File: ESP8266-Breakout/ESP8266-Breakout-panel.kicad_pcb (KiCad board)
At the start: 2 copper layers, 98.8 x 97.2 mm, 258 parts, among them J101 Conn_01x09_Female, J102 Conn_01x09_Female, J501 FTDI, SW501 Flash, SW502 RST, U101 AMS1117-3.3, U501 ESP-12F

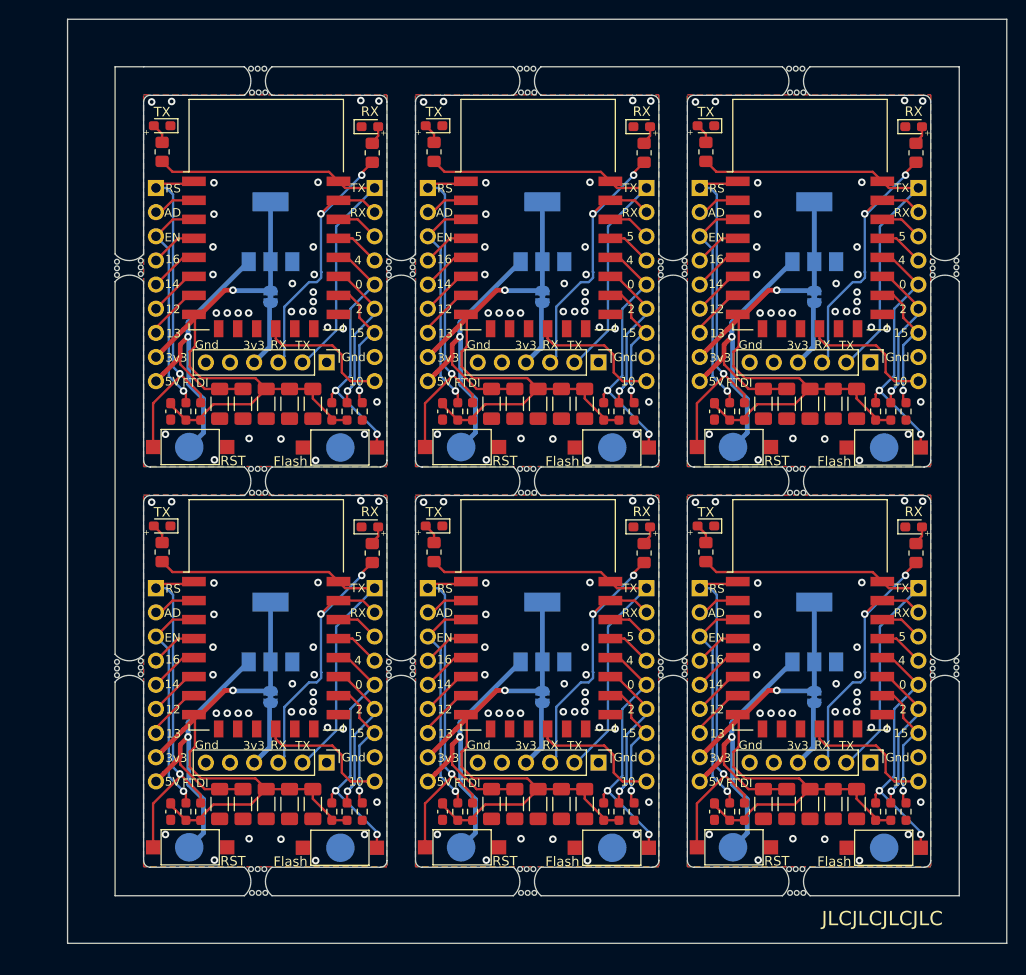
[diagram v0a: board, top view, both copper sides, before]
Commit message: Release 2
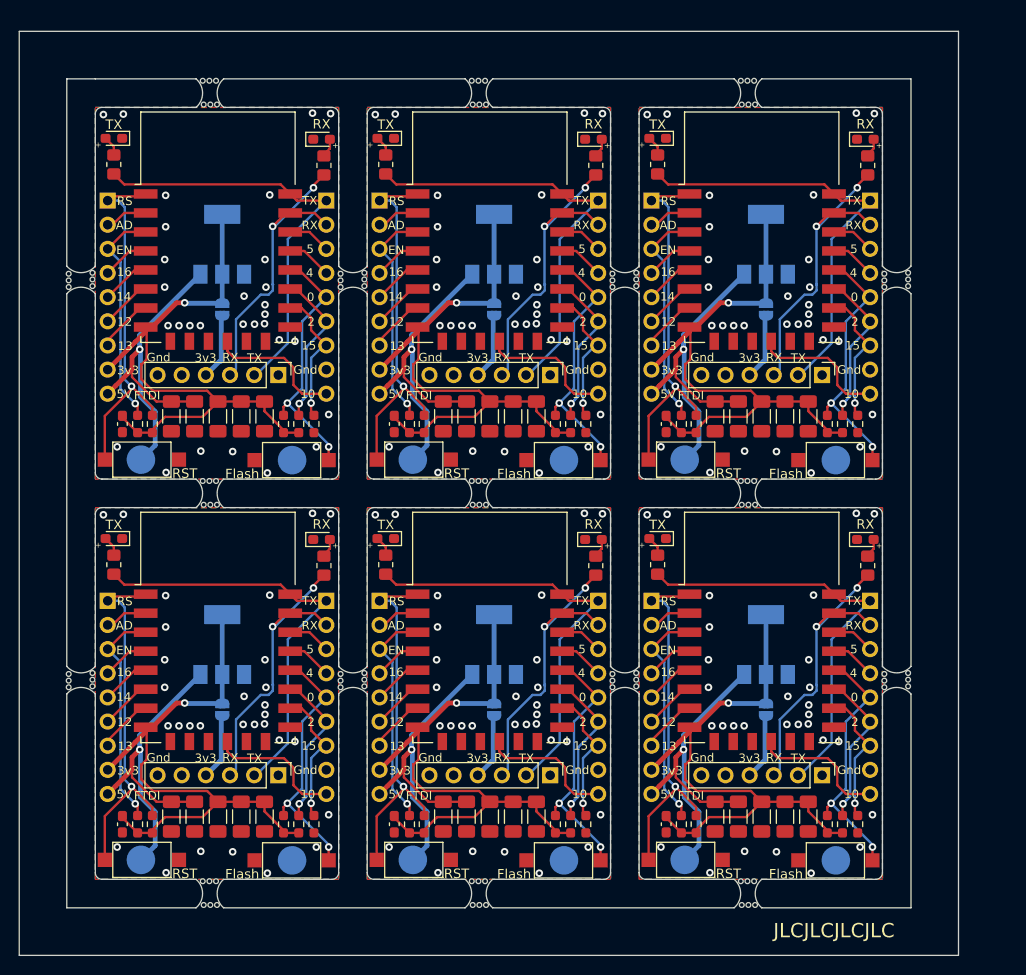
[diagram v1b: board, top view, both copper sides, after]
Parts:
- removed the C101 at (177.6, 129.2)
- removed the C101 at (148.9, 129.2)
- removed the C101 at (120.3, 129.2)
- removed the C101 at (177.6, 87.0)
- removed the C101 at (148.9, 87.0)
- removed the C101 at (120.3, 87.0)
- removed the C102 at (175.1, 129.2)
- removed the C102 at (146.5, 129.2)
- removed the C102 at (117.9, 129.2)
- removed the C102 at (175.1, 87.0)
- removed the C102 at (146.5, 87.0)
- removed the C102 at (117.9, 87.0)
- removed the C103 at (182.4, 129.2)
- removed the C103 at (153.8, 129.2)
- removed the C103 at (125.2, 129.2)
- removed the C103 at (182.4, 87.0)
- removed the C103 at (153.8, 87.0)
- removed the C103 at (125.2, 87.0)
- removed the C104 at (184.9, 129.2)
- removed the C104 at (156.3, 129.2)
- removed the C104 at (127.7, 129.2)
- removed the C104 at (184.9, 87.0)
- removed the C104 at (156.3, 87.0)
- removed the C104 at (127.7, 87.0)
- removed the C501 at (169.9, 129.9)
- removed the C501 at (141.3, 129.9)
- removed the C501 at (112.8, 129.9)
- removed the C501 at (169.9, 87.8)
- removed the C501 at (141.3, 87.8)
- removed the C501 at (112.8, 87.8)
- removed the C502 at (180.0, 129.2)
- removed the C502 at (151.4, 129.2)
- removed the C502 at (122.8, 129.2)
- removed the C502 at (180.0, 87.0)
- removed the C502 at (151.4, 87.0)
- removed the C502 at (122.8, 87.0)
- removed the D501 at (169.1, 99.9)
- removed the D501 at (140.4, 99.9)
- removed the D501 at (111.8, 99.9)
- removed the D501 at (169.1, 57.8)
- removed the D501 at (140.4, 57.8)
- removed the D501 at (111.8, 57.8)
- removed the D502 at (190.9, 100.0)
- removed the D502 at (162.3, 100.0)
- removed the D502 at (133.7, 100.0)
- removed the D502 at (190.9, 57.9)
- removed the D502 at (162.3, 57.9)
- removed the D502 at (133.7, 57.9)
- removed the J101 at (168.4, 106.5)
- removed the J101 at (139.8, 106.5)
- removed the J101 at (111.2, 106.5)
- removed the J101 at (168.4, 64.3)
- removed the J101 at (139.8, 64.3)
- removed the J101 at (111.2, 64.3)
- removed the J102 at (191.4, 106.5)
- removed the J102 at (162.8, 106.5)
- removed the J102 at (134.2, 106.5)
- removed the J102 at (191.4, 64.3)
- removed the J102 at (162.8, 64.3)
- removed the J102 at (134.2, 64.3)
- removed the J501 at (186.3, 124.8)
- removed the J501 at (157.8, 124.8)
- removed the J501 at (129.2, 124.8)
- removed the J501 at (186.3, 82.7)
- removed the J501 at (157.8, 82.7)
- removed the J501 at (129.2, 82.7)
- removed the JP501 at (180.4, 117.9)
- removed the JP501 at (151.8, 117.9)
- removed the JP501 at (123.2, 117.9)
- removed the JP501 at (180.4, 75.8)
- removed the JP501 at (151.8, 75.8)
- removed the JP501 at (123.2, 75.8)
- removed the R501 at (186.9, 129.9)
- removed the R501 at (158.3, 129.9)
- removed the R501 at (129.7, 129.9)
- removed the R501 at (186.9, 87.8)
- removed the R501 at (158.3, 87.8)
- removed the R501 at (129.7, 87.8)
- removed the R502 at (173.1, 129.9)
- removed the R502 at (144.5, 129.9)
- removed the R502 at (115.9, 129.9)
- removed the R502 at (173.1, 87.8)
- removed the R502 at (144.5, 87.8)
- removed the R502 at (115.9, 87.8)
- removed the R503 at (171.6, 129.9)
- removed the R503 at (142.9, 129.9)
- removed the R503 at (114.3, 129.9)
- removed the R503 at (171.6, 87.8)
- removed the R503 at (142.9, 87.8)
- removed the R503 at (114.3, 87.8)
- removed the R504 at (169.1, 102.7)
- removed the R504 at (140.4, 102.7)
- removed the R504 at (111.8, 102.7)
- removed the R504 at (169.1, 60.5)
- removed the R504 at (140.4, 60.5)
- removed the R504 at (111.8, 60.5)
- removed the R505 at (188.5, 129.9)
- removed the R505 at (159.9, 129.9)
- removed the R505 at (131.3, 129.9)
- removed the R505 at (188.5, 87.8)
- removed the R505 at (159.9, 87.8)
- removed the R505 at (131.3, 87.8)
- removed the R506 at (190.1, 129.9)
- removed the R506 at (161.5, 129.9)
- removed the R506 at (132.9, 129.9)
- removed the R506 at (190.1, 87.8)
- removed the R506 at (161.5, 87.8)
- removed the R506 at (132.9, 87.8)
- removed the R507 at (191.2, 102.8)
- removed the R507 at (162.6, 102.8)
- removed the R507 at (133.9, 102.8)
- removed the R507 at (191.2, 60.6)
- removed the R507 at (162.6, 60.6)
- removed the R507 at (133.9, 60.6)
- removed the REF** at (179.9, 100.3)
- removed the REF** at (109.6, 115.5)
- removed the REF** at (121.3, 96.4)
- removed the REF** at (177.9, 54.3)
- removed the REF** at (149.6, 54.3)
- removed the REF** at (122.0, 54.3)
- removed the REF** at (122.7, 54.3)
- removed the REF** at (121.3, 54.3)
- removed the REF** at (122.6, 51.8)
- removed the REF** at (121.9, 51.8)
- removed the REF** at (121.2, 51.8)
- removed the REF** at (195.4, 73.4)
- removed the REF** at (166.8, 73.4)
- removed the REF** at (138.2, 73.4)
- removed the REF** at (192.9, 115.6)
- removed the REF** at (164.3, 115.6)
- removed the REF** at (135.7, 115.6)
- removed the REF** at (107.1, 115.6)
- removed the REF** at (192.9, 73.5)
- removed the REF** at (164.3, 73.5)
- removed the REF** at (151.3, 100.3)
- removed the REF** at (135.7, 73.5)
- removed the REF** at (192.9, 114.9)
- removed the REF** at (164.3, 114.9)
- removed the REF** at (135.7, 114.9)
- removed the REF** at (107.1, 114.9)
- removed the REF** at (192.9, 72.8)
- removed the REF** at (164.3, 72.8)
- removed the REF** at (135.7, 72.8)
- removed the REF** at (192.9, 114.2)
- removed the REF** at (164.3, 114.2)
- removed the REF** at (122.7, 100.3)
- removed the REF** at (135.7, 114.2)
- removed the REF** at (107.1, 114.2)
- removed the REF** at (192.9, 72.1)
- removed the REF** at (164.3, 72.1)
- removed the REF** at (135.7, 72.1)
- removed the REF** at (195.4, 114.1)
- removed the REF** at (166.8, 114.1)
- removed the REF** at (138.2, 114.1)
- removed the REF** at (109.6, 114.1)
- removed the REF** at (195.4, 72.0)
- removed the REF** at (179.9, 58.2)
- removed the REF** at (166.8, 72.0)
- removed the REF** at (138.2, 72.0)
- removed the REF** at (195.4, 114.8)
- removed the REF** at (166.8, 114.8)
- removed the REF** at (138.2, 114.8)
- removed the REF** at (109.6, 114.8)
- removed the REF** at (195.4, 72.7)
- removed the REF** at (166.8, 72.7)
- removed the REF** at (138.2, 72.7)
- removed the REF** at (109.6, 72.7)
- removed the REF** at (151.3, 58.2)
- removed the REF** at (109.6, 72.0)
- removed the REF** at (107.1, 72.8)
- removed the REF** at (107.1, 72.1)
- removed the REF** at (107.1, 73.5)
- removed the REF** at (109.6, 73.4)
- removed the REF** at (178.6, 138.5)
- removed the REF** at (150.3, 138.5)
- removed the REF** at (122.0, 138.5)
- removed the REF** at (178.6, 96.4)
- removed the REF** at (150.3, 96.4)
- removed the REF** at (122.7, 58.2)
- removed the REF** at (122.0, 96.4)
- removed the REF** at (178.6, 54.3)
- removed the REF** at (150.3, 54.3)
- removed the REF** at (179.3, 138.5)
- removed the REF** at (151.0, 138.5)
- removed the REF** at (122.7, 138.5)
- removed the REF** at (179.3, 96.4)
- removed the REF** at (151.0, 96.4)
- removed the REF** at (122.7, 96.4)
- removed the REF** at (179.3, 54.3)
- removed the REF** at (195.4, 115.5)
- removed the REF** at (151.0, 54.3)
- removed the REF** at (178.5, 136.0)
- removed the REF** at (150.2, 136.0)
- removed the REF** at (121.9, 136.0)
- removed the REF** at (178.5, 93.9)
- removed the REF** at (150.2, 93.9)
- removed the REF** at (121.9, 93.9)
- removed the REF** at (178.5, 51.8)
- removed the REF** at (150.2, 51.8)
- removed the REF** at (179.2, 136.0)
- removed the REF** at (166.8, 115.5)
- removed the REF** at (150.9, 136.0)
- removed the REF** at (122.6, 136.0)
- removed the REF** at (179.2, 93.9)
- removed the REF** at (150.9, 93.9)
- removed the REF** at (122.6, 93.9)
- removed the REF** at (179.2, 51.8)
- removed the REF** at (150.9, 51.8)
- removed the REF** at (177.8, 136.0)
- removed the REF** at (149.5, 136.0)
- removed the REF** at (121.2, 136.0)
- removed the REF** at (138.2, 115.5)
- removed the REF** at (177.8, 93.9)
- removed the REF** at (149.5, 93.9)
- removed the REF** at (121.2, 93.9)
- removed the REF** at (177.8, 51.8)
- removed the REF** at (149.5, 51.8)
- removed the REF** at (177.9, 138.5)
- removed the REF** at (149.6, 138.5)
- removed the REF** at (121.3, 138.5)
- removed the REF** at (177.9, 96.4)
- removed the REF** at (149.6, 96.4)
- removed the SW501 at (187.8, 133.8)
- removed the SW501 at (159.2, 133.8)
- removed the SW501 at (130.6, 133.8)
- removed the SW501 at (187.8, 91.7)
- removed the SW501 at (159.2, 91.7)
- removed the SW501 at (130.6, 91.7)
- removed the SW502 at (172.0, 133.7)
- removed the SW502 at (143.4, 133.7)
- removed the SW502 at (114.8, 133.7)
- removed the SW502 at (172.0, 91.6)
- removed the SW502 at (143.4, 91.6)
- removed the SW502 at (114.8, 91.6)
- removed the TP101 at (171.9, 133.7)
- removed the TP101 at (143.3, 133.7)
- removed the TP101 at (114.7, 133.7)
- removed the TP101 at (171.9, 91.6)
- removed the TP101 at (143.3, 91.6)
- removed the TP101 at (114.7, 91.6)
- removed the TP102 at (187.8, 133.8)
- removed the TP102 at (159.2, 133.8)
- removed the TP102 at (130.6, 133.8)
- removed the TP102 at (187.8, 91.7)
- removed the TP102 at (159.2, 91.7)
- removed the TP102 at (130.6, 91.7)
- removed the U101 at (180.4, 111.0)
- removed the U101 at (151.8, 111.0)
- removed the U101 at (123.2, 111.0)
- removed the U101 at (180.4, 69.0)
- removed the U101 at (151.8, 69.0)
- removed the U101 at (123.2, 69.0)
- removed the U501 at (180.0, 109.2)
- removed the U501 at (151.4, 109.2)
- removed the U501 at (122.8, 109.2)
- removed the U501 at (180.0, 67.2)
- removed the U501 at (151.4, 67.2)
- removed the U501 at (122.8, 67.2)
- added C101: 10uF, Capacitor_SMD:C_1206_3216Metric_Pad1.33x1.80mm_HandSolder, F.Cu at (172.5, 130.5)
- added C101: 10uF, Capacitor_SMD:C_1206_3216Metric_Pad1.33x1.80mm_HandSolder, F.Cu at (143.9, 130.5)
- added C101: 10uF, Capacitor_SMD:C_1206_3216Metric_Pad1.33x1.80mm_HandSolder, F.Cu at (115.3, 130.5)
- added C101: 10uF, Capacitor_SMD:C_1206_3216Metric_Pad1.33x1.80mm_HandSolder, F.Cu at (172.5, 88.4)
- added C101: 10uF, Capacitor_SMD:C_1206_3216Metric_Pad1.33x1.80mm_HandSolder, F.Cu at (143.9, 88.4)
- added C101: 10uF, Capacitor_SMD:C_1206_3216Metric_Pad1.33x1.80mm_HandSolder, F.Cu at (115.3, 88.4)
- added C102: 100nF, Capacitor_SMD:C_1206_3216Metric_Pad1.33x1.80mm_HandSolder, F.Cu at (170.0, 130.5)
- added C102: 100nF, Capacitor_SMD:C_1206_3216Metric_Pad1.33x1.80mm_HandSolder, F.Cu at (141.4, 130.5)
- added C102: 100nF, Capacitor_SMD:C_1206_3216Metric_Pad1.33x1.80mm_HandSolder, F.Cu at (112.8, 130.5)
- added C102: 100nF, Capacitor_SMD:C_1206_3216Metric_Pad1.33x1.80mm_HandSolder, F.Cu at (170.0, 88.4)
- added C102: 100nF, Capacitor_SMD:C_1206_3216Metric_Pad1.33x1.80mm_HandSolder, F.Cu at (141.4, 88.4)
- added C102: 100nF, Capacitor_SMD:C_1206_3216Metric_Pad1.33x1.80mm_HandSolder, F.Cu at (112.8, 88.4)
- added C103: 100nF, Capacitor_SMD:C_1206_3216Metric_Pad1.33x1.80mm_HandSolder, F.Cu at (177.4, 130.5)
- added C103: 100nF, Capacitor_SMD:C_1206_3216Metric_Pad1.33x1.80mm_HandSolder, F.Cu at (148.8, 130.5)
- added C103: 100nF, Capacitor_SMD:C_1206_3216Metric_Pad1.33x1.80mm_HandSolder, F.Cu at (120.2, 130.5)
- added C103: 100nF, Capacitor_SMD:C_1206_3216Metric_Pad1.33x1.80mm_HandSolder, F.Cu at (177.4, 88.4)
- added C103: 100nF, Capacitor_SMD:C_1206_3216Metric_Pad1.33x1.80mm_HandSolder, F.Cu at (148.8, 88.4)
- added C103: 100nF, Capacitor_SMD:C_1206_3216Metric_Pad1.33x1.80mm_HandSolder, F.Cu at (120.2, 88.4)
- added C104: 10uF, Capacitor_SMD:C_1206_3216Metric_Pad1.33x1.80mm_HandSolder, F.Cu at (179.8, 130.5)
- added C104: 10uF, Capacitor_SMD:C_1206_3216Metric_Pad1.33x1.80mm_HandSolder, F.Cu at (151.2, 130.5)
- added C104: 10uF, Capacitor_SMD:C_1206_3216Metric_Pad1.33x1.80mm_HandSolder, F.Cu at (122.6, 130.5)
- added C104: 10uF, Capacitor_SMD:C_1206_3216Metric_Pad1.33x1.80mm_HandSolder, F.Cu at (179.8, 88.4)
- added C104: 10uF, Capacitor_SMD:C_1206_3216Metric_Pad1.33x1.80mm_HandSolder, F.Cu at (151.2, 88.4)
- added C104: 10uF, Capacitor_SMD:C_1206_3216Metric_Pad1.33x1.80mm_HandSolder, F.Cu at (122.6, 88.4)
- added C501: 0.1uF, Capacitor_SMD:C_0603_1608Metric_Pad1.08x0.95mm_HandSolder, F.Cu at (164.9, 131.3)
- added C501: 0.1uF, Capacitor_SMD:C_0603_1608Metric_Pad1.08x0.95mm_HandSolder, F.Cu at (136.3, 131.3)
- added C501: 0.1uF, Capacitor_SMD:C_0603_1608Metric_Pad1.08x0.95mm_HandSolder, F.Cu at (107.7, 131.3)
- added C501: 0.1uF, Capacitor_SMD:C_0603_1608Metric_Pad1.08x0.95mm_HandSolder, F.Cu at (164.9, 89.2)
- added C501: 0.1uF, Capacitor_SMD:C_0603_1608Metric_Pad1.08x0.95mm_HandSolder, F.Cu at (136.3, 89.2)
- added C501: 0.1uF, Capacitor_SMD:C_0603_1608Metric_Pad1.08x0.95mm_HandSolder, F.Cu at (107.7, 89.2)
- added C502: 47uF, Capacitor_SMD:C_1206_3216Metric_Pad1.33x1.80mm_HandSolder, F.Cu at (174.9, 130.5)
- added C502: 47uF, Capacitor_SMD:C_1206_3216Metric_Pad1.33x1.80mm_HandSolder, F.Cu at (146.3, 130.5)
- added C502: 47uF, Capacitor_SMD:C_1206_3216Metric_Pad1.33x1.80mm_HandSolder, F.Cu at (117.7, 130.5)
- added C502: 47uF, Capacitor_SMD:C_1206_3216Metric_Pad1.33x1.80mm_HandSolder, F.Cu at (174.9, 88.4)
- added C502: 47uF, Capacitor_SMD:C_1206_3216Metric_Pad1.33x1.80mm_HandSolder, F.Cu at (146.3, 88.4)
- added C502: 47uF, Capacitor_SMD:C_1206_3216Metric_Pad1.33x1.80mm_HandSolder, F.Cu at (117.7, 88.4)
- added D501: TX, LED_SMD:LED_0603_1608Metric_Pad1.05x0.95mm_HandSolder, F.Cu at (164.0, 101.2)
- added D501: TX, LED_SMD:LED_0603_1608Metric_Pad1.05x0.95mm_HandSolder, F.Cu at (135.4, 101.2)
- added D501: TX, LED_SMD:LED_0603_1608Metric_Pad1.05x0.95mm_HandSolder, F.Cu at (106.8, 101.2)
- added D501: TX, LED_SMD:LED_0603_1608Metric_Pad1.05x0.95mm_HandSolder, F.Cu at (164.0, 59.1)
- added D501: TX, LED_SMD:LED_0603_1608Metric_Pad1.05x0.95mm_HandSolder, F.Cu at (135.4, 59.1)
- added D501: TX, LED_SMD:LED_0603_1608Metric_Pad1.05x0.95mm_HandSolder, F.Cu at (106.8, 59.1)
- added D502: RX, LED_SMD:LED_0603_1608Metric_Pad1.05x0.95mm_HandSolder, F.Cu at (185.8, 101.3)
- added D502: RX, LED_SMD:LED_0603_1608Metric_Pad1.05x0.95mm_HandSolder, F.Cu at (157.2, 101.3)
- added D502: RX, LED_SMD:LED_0603_1608Metric_Pad1.05x0.95mm_HandSolder, F.Cu at (128.6, 101.3)
- added D502: RX, LED_SMD:LED_0603_1608Metric_Pad1.05x0.95mm_HandSolder, F.Cu at (185.8, 59.2)
- added D502: RX, LED_SMD:LED_0603_1608Metric_Pad1.05x0.95mm_HandSolder, F.Cu at (157.2, 59.2)
- added D502: RX, LED_SMD:LED_0603_1608Metric_Pad1.05x0.95mm_HandSolder, F.Cu at (128.6, 59.2)
- added J101: Conn_01x09_Female, Custom:PinHeader_1x09_P2.54mm_Vertical_without_silkscrean, F.Cu at (163.3, 107.8)
- added J101: Conn_01x09_Female, Custom:PinHeader_1x09_P2.54mm_Vertical_without_silkscrean, F.Cu at (134.7, 107.8)
- added J101: Conn_01x09_Female, Custom:PinHeader_1x09_P2.54mm_Vertical_without_silkscrean, F.Cu at (106.1, 107.8)
- added J101: Conn_01x09_Female, Custom:PinHeader_1x09_P2.54mm_Vertical_without_silkscrean, F.Cu at (163.3, 65.7)
- added J101: Conn_01x09_Female, Custom:PinHeader_1x09_P2.54mm_Vertical_without_silkscrean, F.Cu at (134.7, 65.7)
- added J101: Conn_01x09_Female, Custom:PinHeader_1x09_P2.54mm_Vertical_without_silkscrean, F.Cu at (106.1, 65.7)
- added J102: Conn_01x09_Female, Custom:PinHeader_1x09_P2.54mm_Vertical_without_silkscrean, F.Cu at (186.3, 107.8)
- added J102: Conn_01x09_Female, Custom:PinHeader_1x09_P2.54mm_Vertical_without_silkscrean, F.Cu at (157.7, 107.8)
- added J102: Conn_01x09_Female, Custom:PinHeader_1x09_P2.54mm_Vertical_without_silkscrean, F.Cu at (129.1, 107.8)
- added J102: Conn_01x09_Female, Custom:PinHeader_1x09_P2.54mm_Vertical_without_silkscrean, F.Cu at (186.3, 65.7)
- added J102: Conn_01x09_Female, Custom:PinHeader_1x09_P2.54mm_Vertical_without_silkscrean, F.Cu at (157.7, 65.7)
- added J102: Conn_01x09_Female, Custom:PinHeader_1x09_P2.54mm_Vertical_without_silkscrean, F.Cu at (129.1, 65.7)
- added J501: FTDI, Connector_PinHeader_2.54mm:PinHeader_1x06_P2.54mm_Vertical, F.Cu at (181.3, 126.1)
- added J501: FTDI, Connector_PinHeader_2.54mm:PinHeader_1x06_P2.54mm_Vertical, F.Cu at (152.7, 126.1)
- added J501: FTDI, Connector_PinHeader_2.54mm:PinHeader_1x06_P2.54mm_Vertical, F.Cu at (124.1, 126.1)
- added J501: FTDI, Connector_PinHeader_2.54mm:PinHeader_1x06_P2.54mm_Vertical, F.Cu at (181.3, 84.0)
- added J501: FTDI, Connector_PinHeader_2.54mm:PinHeader_1x06_P2.54mm_Vertical, F.Cu at (152.7, 84.0)
- added J501: FTDI, Connector_PinHeader_2.54mm:PinHeader_1x06_P2.54mm_Vertical, F.Cu at (124.1, 84.0)
- added JP501: Power, Jumper:SolderJumper-2_P1.3mm_Open_RoundedPad1.0x1.5mm, B.Cu at (175.4, 119.2)
- added JP501: Power, Jumper:SolderJumper-2_P1.3mm_Open_RoundedPad1.0x1.5mm, B.Cu at (146.8, 119.2)
- added JP501: Power, Jumper:SolderJumper-2_P1.3mm_Open_RoundedPad1.0x1.5mm, B.Cu at (118.2, 119.2)
- added JP501: Power, Jumper:SolderJumper-2_P1.3mm_Open_RoundedPad1.0x1.5mm, B.Cu at (175.4, 77.1)
- added JP501: Power, Jumper:SolderJumper-2_P1.3mm_Open_RoundedPad1.0x1.5mm, B.Cu at (146.8, 77.1)
- added JP501: Power, Jumper:SolderJumper-2_P1.3mm_Open_RoundedPad1.0x1.5mm, B.Cu at (118.2, 77.1)
- added R501: 10K, Resistor_SMD:R_0603_1608Metric_Pad0.98x0.95mm_HandSolder, F.Cu at (181.8, 131.3)
- added R501: 10K, Resistor_SMD:R_0603_1608Metric_Pad0.98x0.95mm_HandSolder, F.Cu at (153.2, 131.3)
- added R501: 10K, Resistor_SMD:R_0603_1608Metric_Pad0.98x0.95mm_HandSolder, F.Cu at (124.6, 131.3)
- added R501: 10K, Resistor_SMD:R_0603_1608Metric_Pad0.98x0.95mm_HandSolder, F.Cu at (181.8, 89.2)
- added R501: 10K, Resistor_SMD:R_0603_1608Metric_Pad0.98x0.95mm_HandSolder, F.Cu at (153.2, 89.2)
- added R501: 10K, Resistor_SMD:R_0603_1608Metric_Pad0.98x0.95mm_HandSolder, F.Cu at (124.6, 89.2)
- added R502: 10K, Resistor_SMD:R_0603_1608Metric_Pad0.98x0.95mm_HandSolder, F.Cu at (168.0, 131.3)
- added R502: 10K, Resistor_SMD:R_0603_1608Metric_Pad0.98x0.95mm_HandSolder, F.Cu at (139.4, 131.3)
- added R502: 10K, Resistor_SMD:R_0603_1608Metric_Pad0.98x0.95mm_HandSolder, F.Cu at (110.8, 131.3)
- added R502: 10K, Resistor_SMD:R_0603_1608Metric_Pad0.98x0.95mm_HandSolder, F.Cu at (168.0, 89.2)
- added R502: 10K, Resistor_SMD:R_0603_1608Metric_Pad0.98x0.95mm_HandSolder, F.Cu at (139.4, 89.2)
- added R502: 10K, Resistor_SMD:R_0603_1608Metric_Pad0.98x0.95mm_HandSolder, F.Cu at (110.8, 89.2)
- added R503: 10K, Resistor_SMD:R_0603_1608Metric_Pad0.98x0.95mm_HandSolder, F.Cu at (166.5, 131.3)
- added R503: 10K, Resistor_SMD:R_0603_1608Metric_Pad0.98x0.95mm_HandSolder, F.Cu at (137.9, 131.3)
- added R503: 10K, Resistor_SMD:R_0603_1608Metric_Pad0.98x0.95mm_HandSolder, F.Cu at (109.3, 131.3)
- added R503: 10K, Resistor_SMD:R_0603_1608Metric_Pad0.98x0.95mm_HandSolder, F.Cu at (166.5, 89.2)
- added R503: 10K, Resistor_SMD:R_0603_1608Metric_Pad0.98x0.95mm_HandSolder, F.Cu at (137.9, 89.2)
- added R503: 10K, Resistor_SMD:R_0603_1608Metric_Pad0.98x0.95mm_HandSolder, F.Cu at (109.3, 89.2)
- added R504: 15, Resistor_SMD:R_0805_2012Metric_Pad1.20x1.40mm_HandSolder, F.Cu at (164.0, 104.0)
- added R504: 15, Resistor_SMD:R_0805_2012Metric_Pad1.20x1.40mm_HandSolder, F.Cu at (135.4, 104.0)
- added R504: 15, Resistor_SMD:R_0805_2012Metric_Pad1.20x1.40mm_HandSolder, F.Cu at (106.8, 104.0)
- added R504: 15, Resistor_SMD:R_0805_2012Metric_Pad1.20x1.40mm_HandSolder, F.Cu at (164.0, 61.9)
- added R504: 15, Resistor_SMD:R_0805_2012Metric_Pad1.20x1.40mm_HandSolder, F.Cu at (135.4, 61.9)
- added R504: 15, Resistor_SMD:R_0805_2012Metric_Pad1.20x1.40mm_HandSolder, F.Cu at (106.8, 61.9)
- added R505: 10K, Resistor_SMD:R_0603_1608Metric_Pad0.98x0.95mm_HandSolder, F.Cu at (183.4, 131.3)
- added R505: 10K, Resistor_SMD:R_0603_1608Metric_Pad0.98x0.95mm_HandSolder, F.Cu at (154.8, 131.3)
- added R505: 10K, Resistor_SMD:R_0603_1608Metric_Pad0.98x0.95mm_HandSolder, F.Cu at (126.2, 131.3)
- added R505: 10K, Resistor_SMD:R_0603_1608Metric_Pad0.98x0.95mm_HandSolder, F.Cu at (183.4, 89.2)
- added R505: 10K, Resistor_SMD:R_0603_1608Metric_Pad0.98x0.95mm_HandSolder, F.Cu at (154.8, 89.2)
- added R505: 10K, Resistor_SMD:R_0603_1608Metric_Pad0.98x0.95mm_HandSolder, F.Cu at (126.2, 89.2)
- added R506: 10K, Resistor_SMD:R_0603_1608Metric_Pad0.98x0.95mm_HandSolder, F.Cu at (185.0, 131.3)
- added R506: 10K, Resistor_SMD:R_0603_1608Metric_Pad0.98x0.95mm_HandSolder, F.Cu at (156.4, 131.3)
- added R506: 10K, Resistor_SMD:R_0603_1608Metric_Pad0.98x0.95mm_HandSolder, F.Cu at (127.8, 131.3)
- added R506: 10K, Resistor_SMD:R_0603_1608Metric_Pad0.98x0.95mm_HandSolder, F.Cu at (185.0, 89.2)
- added R506: 10K, Resistor_SMD:R_0603_1608Metric_Pad0.98x0.95mm_HandSolder, F.Cu at (156.4, 89.2)
- added R506: 10K, Resistor_SMD:R_0603_1608Metric_Pad0.98x0.95mm_HandSolder, F.Cu at (127.8, 89.2)
- added R507: 15, Resistor_SMD:R_0805_2012Metric_Pad1.20x1.40mm_HandSolder, F.Cu at (186.1, 104.1)
- added R507: 15, Resistor_SMD:R_0805_2012Metric_Pad1.20x1.40mm_HandSolder, F.Cu at (157.5, 104.1)
- added R507: 15, Resistor_SMD:R_0805_2012Metric_Pad1.20x1.40mm_HandSolder, F.Cu at (128.9, 104.1)
- added R507: 15, Resistor_SMD:R_0805_2012Metric_Pad1.20x1.40mm_HandSolder, F.Cu at (186.1, 62.0)
- added R507: 15, Resistor_SMD:R_0805_2012Metric_Pad1.20x1.40mm_HandSolder, F.Cu at (157.5, 62.0)
- added R507: 15, Resistor_SMD:R_0805_2012Metric_Pad1.20x1.40mm_HandSolder, F.Cu at (128.9, 62.0)
- added REF**: KiCad-Logo_5mm_SilkScreen, Symbol:KiCad-Logo_5mm_SilkScreen, B.Cu at (174.8, 101.6)
- added REF**: 0.5mm-NPTH-Drill, panels:0.5mm-NPTH-Drill, F.Cu at (187.8, 115.5)
- added REF**: 0.5mm-NPTH-Drill, panels:0.5mm-NPTH-Drill, F.Cu at (187.8, 73.4)
- added REF**: 0.5mm-NPTH-Drill, panels:0.5mm-NPTH-Drill, F.Cu at (145.2, 55.6)
- added REF**: 0.5mm-NPTH-Drill, panels:0.5mm-NPTH-Drill, F.Cu at (174.2, 139.8)
- added REF**: 0.5mm-NPTH-Drill, panels:0.5mm-NPTH-Drill, F.Cu at (159.2, 116.2)
- added REF**: 0.5mm-NPTH-Drill, panels:0.5mm-NPTH-Drill, F.Cu at (161.7, 116.8)
- added REF**: 0.5mm-NPTH-Drill, panels:0.5mm-NPTH-Drill, F.Cu at (190.3, 116.8)
- added REF**: 0.5mm-NPTH-Drill, panels:0.5mm-NPTH-Drill, F.Cu at (133.1, 116.8)
- added REF**: 0.5mm-NPTH-Drill, panels:0.5mm-NPTH-Drill, F.Cu at (104.5, 116.8)
- added REF**: 0.5mm-NPTH-Drill, panels:0.5mm-NPTH-Drill, F.Cu at (190.3, 74.7)
- added REF**: 0.5mm-NPTH-Drill, panels:0.5mm-NPTH-Drill, F.Cu at (145.9, 97.7)
- added REF**: 0.5mm-NPTH-Drill, panels:0.5mm-NPTH-Drill, F.Cu at (174.2, 97.7)
- added REF**: 0.5mm-NPTH-Drill, panels:0.5mm-NPTH-Drill, F.Cu at (116.8, 95.2)
- added REF**: 0.5mm-NPTH-Drill, panels:0.5mm-NPTH-Drill, F.Cu at (145.1, 95.2)
- added REF**: 0.5mm-NPTH-Drill, panels:0.5mm-NPTH-Drill, F.Cu at (145.2, 139.8)
- added REF**: 0.5mm-NPTH-Drill, panels:0.5mm-NPTH-Drill, F.Cu at (130.6, 116.9)
- added REF**: 0.5mm-NPTH-Drill, panels:0.5mm-NPTH-Drill, F.Cu at (161.7, 116.1)
- added REF**: 0.5mm-NPTH-Drill, panels:0.5mm-NPTH-Drill, F.Cu at (102.0, 74.8)
- added REF**: 0.5mm-NPTH-Drill, panels:0.5mm-NPTH-Drill, F.Cu at (104.5, 74.0)
- added REF**: KiCad-Logo_5mm_SilkScreen, Symbol:KiCad-Logo_5mm_SilkScreen, B.Cu at (146.2, 101.6)
- added REF**: 0.5mm-NPTH-Drill, panels:0.5mm-NPTH-Drill, F.Cu at (190.3, 74.0)
- added REF**: 0.5mm-NPTH-Drill, panels:0.5mm-NPTH-Drill, F.Cu at (133.1, 116.1)
- added REF**: 0.5mm-NPTH-Drill, panels:0.5mm-NPTH-Drill, F.Cu at (161.7, 74.7)
- added REF**: 0.5mm-NPTH-Drill, panels:0.5mm-NPTH-Drill, F.Cu at (102.0, 74.1)
- added REF**: 0.5mm-NPTH-Drill, panels:0.5mm-NPTH-Drill, F.Cu at (187.8, 116.9)
- added REF**: 0.5mm-NPTH-Drill, panels:0.5mm-NPTH-Drill, F.Cu at (102.0, 73.4)
- added REF**: 0.5mm-NPTH-Drill, panels:0.5mm-NPTH-Drill, F.Cu at (187.8, 74.8)
- added REF**: 0.5mm-NPTH-Drill, panels:0.5mm-NPTH-Drill, F.Cu at (116.9, 139.8)
- added REF**: 0.5mm-NPTH-Drill, panels:0.5mm-NPTH-Drill, F.Cu at (187.8, 116.2)
- added REF**: 0.5mm-NPTH-Drill, panels:0.5mm-NPTH-Drill, F.Cu at (130.6, 74.8)
- added REF**: KiCad-Logo_5mm_SilkScreen, Symbol:KiCad-Logo_5mm_SilkScreen, B.Cu at (117.6, 101.6)
- added REF**: 0.5mm-NPTH-Drill, panels:0.5mm-NPTH-Drill, F.Cu at (104.5, 74.7)
- added REF**: 0.5mm-NPTH-Drill, panels:0.5mm-NPTH-Drill, F.Cu at (104.5, 116.1)
- added REF**: 0.5mm-NPTH-Drill, panels:0.5mm-NPTH-Drill, F.Cu at (133.1, 74.0)
- added REF**: 0.5mm-NPTH-Drill, panels:0.5mm-NPTH-Drill, F.Cu at (145.2, 97.7)
- added REF**: 0.5mm-NPTH-Drill, panels:0.5mm-NPTH-Drill, F.Cu at (133.1, 74.7)
- added REF**: 0.5mm-NPTH-Drill, panels:0.5mm-NPTH-Drill, F.Cu at (159.2, 74.8)
- added REF**: 0.5mm-NPTH-Drill, panels:0.5mm-NPTH-Drill, F.Cu at (173.5, 139.8)
- added REF**: 0.5mm-NPTH-Drill, panels:0.5mm-NPTH-Drill, F.Cu at (130.6, 116.2)
- added REF**: 0.5mm-NPTH-Drill, panels:0.5mm-NPTH-Drill, F.Cu at (161.7, 74.0)
- added REF**: 0.5mm-NPTH-Drill, panels:0.5mm-NPTH-Drill, F.Cu at (104.5, 73.3)
- added REF**: KiCad-Logo_5mm_SilkScreen, Symbol:KiCad-Logo_5mm_SilkScreen, B.Cu at (174.8, 59.5)
- added REF**: 0.5mm-NPTH-Drill, panels:0.5mm-NPTH-Drill, F.Cu at (187.8, 74.1)
- added REF**: 0.5mm-NPTH-Drill, panels:0.5mm-NPTH-Drill, F.Cu at (102.0, 116.2)
- added REF**: 0.5mm-NPTH-Drill, panels:0.5mm-NPTH-Drill, F.Cu at (130.6, 74.1)
- added REF**: 0.5mm-NPTH-Drill, panels:0.5mm-NPTH-Drill, F.Cu at (159.2, 74.1)
- added REF**: 0.5mm-NPTH-Drill, panels:0.5mm-NPTH-Drill, F.Cu at (159.2, 116.9)
- added REF**: 0.5mm-NPTH-Drill, panels:0.5mm-NPTH-Drill, F.Cu at (174.2, 55.6)
- added REF**: 0.5mm-NPTH-Drill, panels:0.5mm-NPTH-Drill, F.Cu at (117.6, 97.7)
- added REF**: 0.5mm-NPTH-Drill, panels:0.5mm-NPTH-Drill, F.Cu at (116.2, 97.7)
- added REF**: 0.5mm-NPTH-Drill, panels:0.5mm-NPTH-Drill, F.Cu at (144.5, 97.7)
- added REF**: 0.5mm-NPTH-Drill, panels:0.5mm-NPTH-Drill, F.Cu at (173.5, 55.6)
- added REF**: KiCad-Logo_5mm_SilkScreen, Symbol:KiCad-Logo_5mm_SilkScreen, B.Cu at (146.2, 59.5)
- added REF**: 0.5mm-NPTH-Drill, panels:0.5mm-NPTH-Drill, F.Cu at (130.6, 73.4)
- added REF**: 0.5mm-NPTH-Drill, panels:0.5mm-NPTH-Drill, F.Cu at (144.5, 55.6)
- added REF**: 0.5mm-NPTH-Drill, panels:0.5mm-NPTH-Drill, F.Cu at (172.8, 55.6)
- added REF**: 0.5mm-NPTH-Drill, panels:0.5mm-NPTH-Drill, F.Cu at (145.1, 137.3)
- added REF**: 0.5mm-NPTH-Drill, panels:0.5mm-NPTH-Drill, F.Cu at (117.6, 55.6)
- added REF**: 0.5mm-NPTH-Drill, panels:0.5mm-NPTH-Drill, F.Cu at (116.9, 55.6)
- added REF**: 0.5mm-NPTH-Drill, panels:0.5mm-NPTH-Drill, F.Cu at (117.5, 53.1)
- added REF**: 0.5mm-NPTH-Drill, panels:0.5mm-NPTH-Drill, F.Cu at (116.2, 55.6)
- added REF**: 0.5mm-NPTH-Drill, panels:0.5mm-NPTH-Drill, F.Cu at (117.6, 139.8)
- added REF**: 0.5mm-NPTH-Drill, panels:0.5mm-NPTH-Drill, F.Cu at (145.9, 139.8)
- added REF**: KiCad-Logo_5mm_SilkScreen, Symbol:KiCad-Logo_5mm_SilkScreen, B.Cu at (117.6, 59.5)
- added REF**: 0.5mm-NPTH-Drill, panels:0.5mm-NPTH-Drill, F.Cu at (173.4, 137.3)
- added REF**: 0.5mm-NPTH-Drill, panels:0.5mm-NPTH-Drill, F.Cu at (145.9, 55.6)
- added REF**: 0.5mm-NPTH-Drill, panels:0.5mm-NPTH-Drill, F.Cu at (145.1, 53.1)
- added REF**: 0.5mm-NPTH-Drill, panels:0.5mm-NPTH-Drill, F.Cu at (173.4, 53.1)
- added REF**: 0.5mm-NPTH-Drill, panels:0.5mm-NPTH-Drill, F.Cu at (117.5, 95.2)
- added REF**: 0.5mm-NPTH-Drill, panels:0.5mm-NPTH-Drill, F.Cu at (145.8, 95.2)
- added REF**: 0.5mm-NPTH-Drill, panels:0.5mm-NPTH-Drill, F.Cu at (116.9, 97.7)
- added REF**: 0.5mm-NPTH-Drill, panels:0.5mm-NPTH-Drill, F.Cu at (159.2, 73.4)
- added REF**: 0.5mm-NPTH-Drill, panels:0.5mm-NPTH-Drill, F.Cu at (145.8, 53.1)
- added REF**: 0.5mm-NPTH-Drill, panels:0.5mm-NPTH-Drill, F.Cu at (174.1, 53.1)
- added REF**: 0.5mm-NPTH-Drill, panels:0.5mm-NPTH-Drill, F.Cu at (159.2, 115.5)
- added REF**: 0.5mm-NPTH-Drill, panels:0.5mm-NPTH-Drill, F.Cu at (144.4, 137.3)
- added REF**: 0.5mm-NPTH-Drill, panels:0.5mm-NPTH-Drill, F.Cu at (172.7, 137.3)
- added REF**: 0.5mm-NPTH-Drill, panels:0.5mm-NPTH-Drill, F.Cu at (130.6, 115.5)
- added REF**: 0.5mm-NPTH-Drill, panels:0.5mm-NPTH-Drill, F.Cu at (172.7, 95.2)
- added REF**: 0.5mm-NPTH-Drill, panels:0.5mm-NPTH-Drill, F.Cu at (116.1, 137.3)
- added REF**: 0.5mm-NPTH-Drill, panels:0.5mm-NPTH-Drill, F.Cu at (190.3, 115.4)
- added REF**: 0.5mm-NPTH-Drill, panels:0.5mm-NPTH-Drill, F.Cu at (116.1, 95.2)
- added REF**: 0.5mm-NPTH-Drill, panels:0.5mm-NPTH-Drill, F.Cu at (144.4, 95.2)
- added REF**: 0.5mm-NPTH-Drill, panels:0.5mm-NPTH-Drill, F.Cu at (144.4, 53.1)
- added REF**: 0.5mm-NPTH-Drill, panels:0.5mm-NPTH-Drill, F.Cu at (172.7, 53.1)
- added REF**: 0.5mm-NPTH-Drill, panels:0.5mm-NPTH-Drill, F.Cu at (102.0, 116.9)
- added REF**: 0.5mm-NPTH-Drill, panels:0.5mm-NPTH-Drill, F.Cu at (144.5, 139.8)
- added REF**: 0.5mm-NPTH-Drill, panels:0.5mm-NPTH-Drill, F.Cu at (172.8, 139.8)
- added REF**: 0.5mm-NPTH-Drill, panels:0.5mm-NPTH-Drill, F.Cu at (161.7, 115.4)
- added REF**: 0.5mm-NPTH-Drill, panels:0.5mm-NPTH-Drill, F.Cu at (116.1, 53.1)
- added REF**: 0.5mm-NPTH-Drill, panels:0.5mm-NPTH-Drill, F.Cu at (116.8, 53.1)
- added REF**: 0.5mm-NPTH-Drill, panels:0.5mm-NPTH-Drill, F.Cu at (133.1, 115.4)
- added REF**: 0.5mm-NPTH-Drill, panels:0.5mm-NPTH-Drill, F.Cu at (104.5, 115.4)
- added REF**: 0.5mm-NPTH-Drill, panels:0.5mm-NPTH-Drill, F.Cu at (190.3, 73.3)
- added REF**: 0.5mm-NPTH-Drill, panels:0.5mm-NPTH-Drill, F.Cu at (172.8, 97.7)
- added REF**: 0.5mm-NPTH-Drill, panels:0.5mm-NPTH-Drill, F.Cu at (116.2, 139.8)
- added REF**: 0.5mm-NPTH-Drill, panels:0.5mm-NPTH-Drill, F.Cu at (173.5, 97.7)
- added REF**: 0.5mm-NPTH-Drill, panels:0.5mm-NPTH-Drill, F.Cu at (174.1, 95.2)
- added REF**: 0.5mm-NPTH-Drill, panels:0.5mm-NPTH-Drill, F.Cu at (117.5, 137.3)
- added REF**: 0.5mm-NPTH-Drill, panels:0.5mm-NPTH-Drill, F.Cu at (102.0, 115.5)
- added REF**: 0.5mm-NPTH-Drill, panels:0.5mm-NPTH-Drill, F.Cu at (161.7, 73.3)
- added REF**: 0.5mm-NPTH-Drill, panels:0.5mm-NPTH-Drill, F.Cu at (145.8, 137.3)
- added REF**: 0.5mm-NPTH-Drill, panels:0.5mm-NPTH-Drill, F.Cu at (174.1, 137.3)
- added REF**: 0.5mm-NPTH-Drill, panels:0.5mm-NPTH-Drill, F.Cu at (133.1, 73.3)
- added REF**: 0.5mm-NPTH-Drill, panels:0.5mm-NPTH-Drill, F.Cu at (190.3, 116.1)
- added REF**: 0.5mm-NPTH-Drill, panels:0.5mm-NPTH-Drill, F.Cu at (173.4, 95.2)
- added REF**: 0.5mm-NPTH-Drill, panels:0.5mm-NPTH-Drill, F.Cu at (116.8, 137.3)
- added SW501: Flash, Button_Switch_SMD:SW_SPST_CK_RS282G05A3, F.Cu at (182.7, 135.1)
- added SW501: Flash, Button_Switch_SMD:SW_SPST_CK_RS282G05A3, F.Cu at (154.1, 135.1)
- added SW501: Flash, Button_Switch_SMD:SW_SPST_CK_RS282G05A3, F.Cu at (125.5, 135.1)
- added SW501: Flash, Button_Switch_SMD:SW_SPST_CK_RS282G05A3, F.Cu at (182.7, 93.0)
- added SW501: Flash, Button_Switch_SMD:SW_SPST_CK_RS282G05A3, F.Cu at (154.1, 93.0)
- added SW501: Flash, Button_Switch_SMD:SW_SPST_CK_RS282G05A3, F.Cu at (125.5, 93.0)
- added SW502: RST, Button_Switch_SMD:SW_SPST_CK_RS282G05A3, F.Cu at (166.9, 135.0)
- added SW502: RST, Button_Switch_SMD:SW_SPST_CK_RS282G05A3, F.Cu at (138.3, 135.0)
- added SW502: RST, Button_Switch_SMD:SW_SPST_CK_RS282G05A3, F.Cu at (109.7, 135.0)
- added SW502: RST, Button_Switch_SMD:SW_SPST_CK_RS282G05A3, F.Cu at (166.9, 92.9)
- added SW502: RST, Button_Switch_SMD:SW_SPST_CK_RS282G05A3, F.Cu at (138.3, 92.9)
- added SW502: RST, Button_Switch_SMD:SW_SPST_CK_RS282G05A3, F.Cu at (109.7, 92.9)
- added TP101: TestPoint, TestPoint:TestPoint_Pad_D3.0mm, B.Cu at (166.8, 135.0)
- added TP101: TestPoint, TestPoint:TestPoint_Pad_D3.0mm, B.Cu at (138.2, 135.0)
- added TP101: TestPoint, TestPoint:TestPoint_Pad_D3.0mm, B.Cu at (109.6, 135.0)
- added TP101: TestPoint, TestPoint:TestPoint_Pad_D3.0mm, B.Cu at (166.8, 92.9)
- added TP101: TestPoint, TestPoint:TestPoint_Pad_D3.0mm, B.Cu at (138.2, 92.9)
- added TP101: TestPoint, TestPoint:TestPoint_Pad_D3.0mm, B.Cu at (109.6, 92.9)
- added TP102: TestPoint, TestPoint:TestPoint_Pad_D3.0mm, B.Cu at (182.7, 135.1)
- added TP102: TestPoint, TestPoint:TestPoint_Pad_D3.0mm, B.Cu at (154.1, 135.1)
- added TP102: TestPoint, TestPoint:TestPoint_Pad_D3.0mm, B.Cu at (125.5, 135.1)
- added TP102: TestPoint, TestPoint:TestPoint_Pad_D3.0mm, B.Cu at (182.7, 93.0)
- added TP102: TestPoint, TestPoint:TestPoint_Pad_D3.0mm, B.Cu at (154.1, 93.0)
- added TP102: TestPoint, TestPoint:TestPoint_Pad_D3.0mm, B.Cu at (125.5, 93.0)
- added U101: AMS1117-3.3, Package_TO_SOT_SMD:SOT-223-3_TabPin2, B.Cu at (175.4, 112.4)
- added U101: AMS1117-3.3, Package_TO_SOT_SMD:SOT-223-3_TabPin2, B.Cu at (146.8, 112.4)
- added U101: AMS1117-3.3, Package_TO_SOT_SMD:SOT-223-3_TabPin2, B.Cu at (118.2, 112.4)
- added U101: AMS1117-3.3, Package_TO_SOT_SMD:SOT-223-3_TabPin2, B.Cu at (175.4, 70.3)
- added U101: AMS1117-3.3, Package_TO_SOT_SMD:SOT-223-3_TabPin2, B.Cu at (146.8, 70.3)
- added U101: AMS1117-3.3, Package_TO_SOT_SMD:SOT-223-3_TabPin2, B.Cu at (118.2, 70.3)
- added U501: ESP-12F, RF_Module:ESP-12E, F.Cu at (174.9, 110.6)
- added U501: ESP-12F, RF_Module:ESP-12E, F.Cu at (146.3, 110.6)
- added U501: ESP-12F, RF_Module:ESP-12E, F.Cu at (117.7, 110.6)
- added U501: ESP-12F, RF_Module:ESP-12E, F.Cu at (174.9, 68.5)
- added U501: ESP-12F, RF_Module:ESP-12E, F.Cu at (146.3, 68.5)
- added U501: ESP-12F, RF_Module:ESP-12E, F.Cu at (117.7, 68.5)
